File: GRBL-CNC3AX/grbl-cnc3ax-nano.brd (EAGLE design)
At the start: 60.6 x 55.9 mm, 6 parts

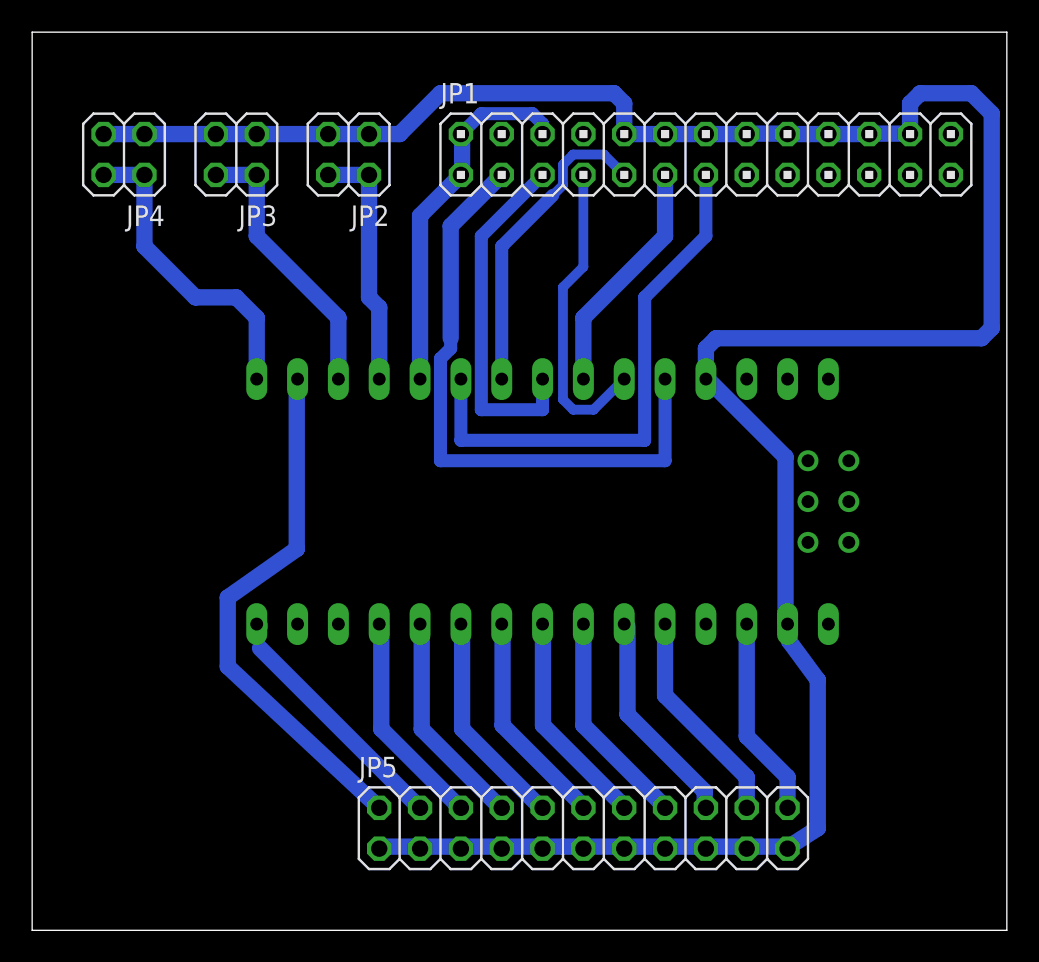
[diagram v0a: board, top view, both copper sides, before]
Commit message: acertos na pcb
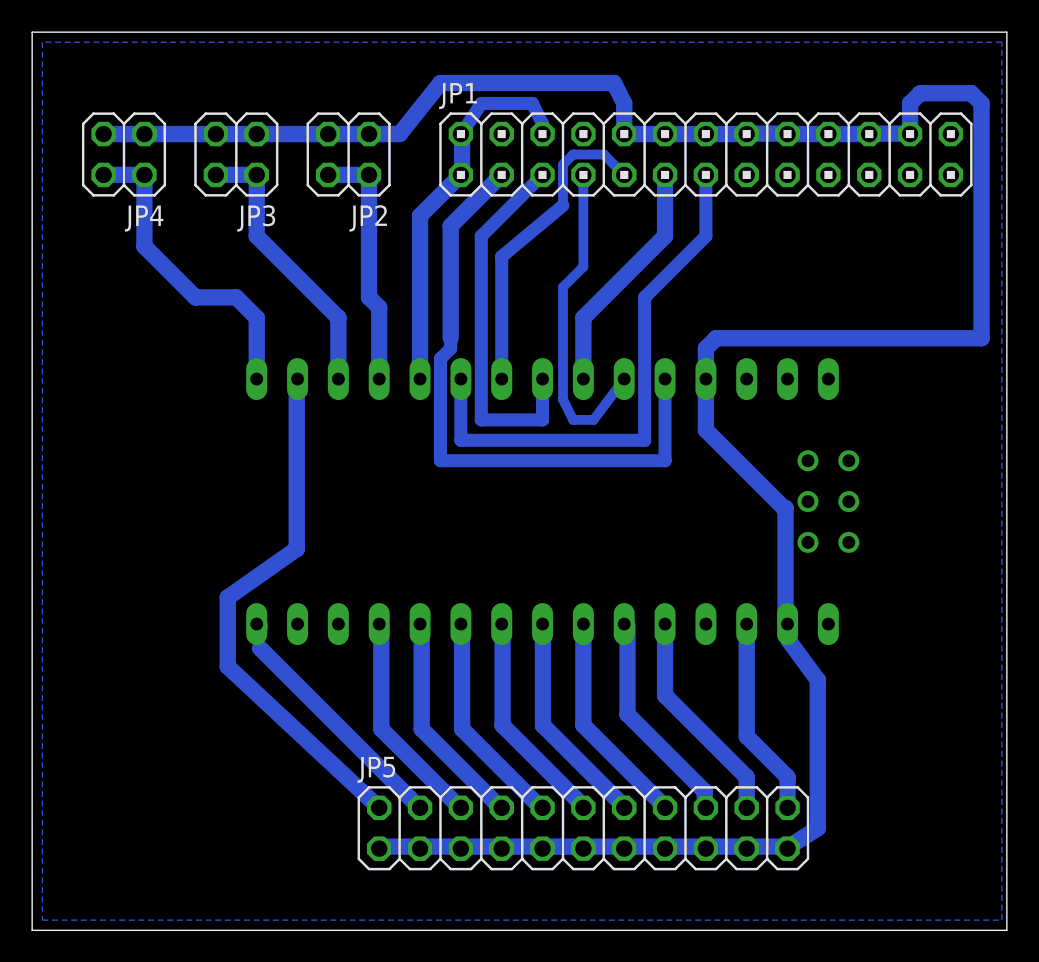
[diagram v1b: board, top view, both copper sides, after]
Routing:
- net X-DIR: track 21.9 -> 23.2 mm
- net ENABLE: track 23.5 -> 24.6 mm
- net Y-STEP: track 19.4 -> 20.4 mm
- added copper zone on layer 16, net N$1
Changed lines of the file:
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@@
 <?xml version="1.0" encoding="utf-8"?>
 <!DOCTYPE eagle SYSTEM "eagle.dtd">
-<eagle version="7.4.0">
+<eagle version="7.2.0">
 <drawing>
 <settings>
@@
 <wire x1="26.7462" y1="54.5338" x2="26.67" y2="54.61" width="1.016" layer="16"/>
 <wire x1="26.7462" y1="54.4068" x2="26.7462" y2="54.6862" width="0.8128" layer="16"/>
-<wire x1="26.7462" y1="54.6862" x2="27.94" y2="55.88" width="0.8128" layer="16"/>
-<wire x1="27.94" y1="55.88" x2="31.115" y2="55.88" width="0.8128" layer="16"/>
-<wire x1="31.115" y1="55.88" x2="31.75" y2="55.245" width="0.8128" layer="16"/>
+<wire x1="26.7462" y1="54.6862" x2="27.94" y2="56.515" width="0.8128" layer="16"/>
+<wire x1="27.94" y1="56.515" x2="31.115" y2="56.515" width="0.8128" layer="16"/>
+<wire x1="31.115" y1="56.515" x2="31.75" y2="55.245" width="0.8128" layer="16"/>
 <wire x1="31.75" y1="55.245" x2="31.75" y2="54.61" width="0.8128" layer="16"/>
 </signal>
@@
 <wire x1="34.29" y1="46.355" x2="33.02" y2="45.085" width="0.6096" layer="16"/>
 <wire x1="33.02" y1="45.085" x2="33.02" y2="38.1" width="0.6096" layer="16"/>
-<wire x1="33.02" y1="38.1" x2="33.655" y2="37.465" width="0.6096" layer="16"/>
-<wire x1="33.655" y1="37.465" x2="34.925" y2="37.465" width="0.6096" layer="16"/>
-<wire x1="34.925" y1="37.465" x2="36.83" y2="39.37" width="0.6096" layer="16"/>
+<wire x1="33.02" y1="38.1" x2="33.655" y2="36.83" width="0.6096" layer="16"/>
+<wire x1="33.655" y1="36.83" x2="34.925" y2="36.83" width="0.6096" layer="16"/>
+<wire x1="34.925" y1="36.83" x2="36.83" y2="39.37" width="0.6096" layer="16"/>
 </signal>
 <signal name="Z-STEP">
@@
 <contactref element="U$1" pad="D5"/>
 <contactref element="JP1" pad="5"/>
-<wire x1="31.75" y1="39.37" x2="31.75" y2="37.465" width="0.8128" layer="16"/>
-<wire x1="31.75" y1="37.465" x2="27.94" y2="37.465" width="0.8128" layer="16"/>
-<wire x1="27.94" y1="37.465" x2="27.94" y2="48.26" width="0.8128" layer="16"/>
+<wire x1="31.75" y1="39.37" x2="31.75" y2="36.83" width="0.8128" layer="16"/>
+<wire x1="31.75" y1="36.83" x2="27.94" y2="36.83" width="0.8128" layer="16"/>
+<wire x1="27.94" y1="36.83" x2="27.94" y2="48.26" width="0.8128" layer="16"/>
 <wire x1="27.94" y1="48.26" x2="31.75" y2="52.07" width="0.8128" layer="16"/>
 </signal>
@@
 <contactref element="U$1" pad="D6"/>
 <contactref element="JP1" pad="9"/>
-<wire x1="29.21" y1="39.37" x2="29.21" y2="47.625" width="0.8128" layer="16"/>
-<wire x1="29.21" y1="47.625" x2="32.385" y2="50.8" width="0.8128" layer="16"/>
-<wire x1="32.385" y1="50.8" x2="33.02" y2="51.435" width="0.6096" layer="16"/>
-<wire x1="33.02" y1="51.435" x2="33.02" y2="52.705" width="0.6096" layer="16"/>
+<wire x1="29.21" y1="39.37" x2="29.21" y2="46.99" width="0.8128" layer="16"/>
+<wire x1="29.21" y1="46.99" x2="33.02" y2="50.165" width="0.8128" layer="16"/>
+<wire x1="33.02" y1="50.165" x2="33.02" y2="52.705" width="0.6096" layer="16"/>
 <wire x1="33.02" y1="52.705" x2="33.655" y2="53.34" width="0.6096" layer="16"/>
 <wire x1="33.655" y1="53.34" x2="35.56" y2="53.34" width="0.6096" layer="16"/>
@@
 <wire x1="46.863" y1="54.6354" x2="46.99" y2="54.61" width="0.254" layer="16"/>
 <wire x1="44.577" y1="54.6354" x2="44.45" y2="54.61" width="0.254" layer="16"/>
-<wire x1="46.863" y1="34.5186" x2="46.863" y2="24.2316" width="1.016" layer="16"/>
-<wire x1="42.0624" y1="39.3192" x2="46.863" y2="34.5186" width="1.016" layer="16"/>
+<wire x1="46.863" y1="31.3436" x2="46.863" y2="24.2316" width="1.016" layer="16"/>
 <wire x1="46.863" y1="24.2316" x2="46.99" y2="24.13" width="0.254" layer="16"/>
-<wire x1="42.0624" y1="39.3192" x2="41.91" y2="39.37" width="0.254" layer="16"/>
 <wire x1="54.4068" y1="54.6354" x2="52.0954" y2="54.6354" width="1.016" layer="16"/>
 <wire x1="52.0954" y1="54.6354" x2="52.07" y2="54.61" width="1.016" layer="16"/>
@@
 <wire x1="41.91" y1="41.275" x2="42.545" y2="41.91" width="1.016" layer="16"/>
 <wire x1="42.545" y1="41.91" x2="59.055" y2="41.91" width="1.016" layer="16"/>
-<wire x1="59.055" y1="41.91" x2="59.69" y2="42.545" width="1.016" layer="16"/>
-<wire x1="59.69" y1="42.545" x2="59.69" y2="55.88" width="1.016" layer="16"/>
-<wire x1="59.69" y1="55.88" x2="58.42" y2="57.15" width="1.016" layer="16"/>
+<wire x1="59.055" y1="41.91" x2="59.055" y2="56.515" width="1.016" layer="16"/>
+<wire x1="59.055" y1="56.515" x2="58.42" y2="57.15" width="1.016" layer="16"/>
 <wire x1="58.42" y1="57.15" x2="55.245" y2="57.15" width="1.016" layer="16"/>
 <wire x1="55.245" y1="57.15" x2="54.61" y2="56.515" width="1.016" layer="16"/>
@@
 <wire x1="18.415" y1="54.61" x2="20.955" y2="54.61" width="1.016" layer="16"/>
 <wire x1="20.955" y1="54.61" x2="22.86" y2="54.61" width="1.016" layer="16"/>
-<wire x1="22.86" y1="54.61" x2="25.4" y2="57.15" width="1.016" layer="16"/>
-<wire x1="25.4" y1="57.15" x2="36.195" y2="57.15" width="1.016" layer="16"/>
-<wire x1="36.195" y1="57.15" x2="36.83" y2="56.515" width="1.016" layer="16"/>
+<wire x1="22.86" y1="54.61" x2="25.4" y2="57.785" width="1.016" layer="16"/>
+<wire x1="25.4" y1="57.785" x2="36.195" y2="57.785" width="1.016" layer="16"/>
+<wire x1="36.195" y1="57.785" x2="36.83" y2="56.515" width="1.016" layer="16"/>
 <wire x1="36.83" y1="56.515" x2="36.83" y2="54.61" width="1.016" layer="16"/>
+<wire x1="46.863" y1="31.3436" x2="46.7614" y2="31.3436" width="1.016" layer="16"/>
+<wire x1="46.7614" y1="31.3436" x2="41.91" y2="36.195" width="1.016" layer="16"/>
+<wire x1="41.91" y1="36.195" x2="41.91" y2="39.37" width="1.016" layer="16"/>
 </signal>
 <signal name="DIR_SPINDLE">
@@
 <wire x1="26.5176" y1="12.8016" x2="26.67" y2="12.7" width="0.254" layer="16"/>
 </signal>
+<signal name="N$1">
+<polygon width="0.4064" layer="16" isolate="1.6764">
+<vertex x="0.635" y="60.325"/>
+<vertex x="0.635" y="5.715"/>
+<vertex x="60.325" y="5.715"/>
+<vertex x="60.325" y="60.325"/>
+</polygon>
+</signal>
 </signals>
